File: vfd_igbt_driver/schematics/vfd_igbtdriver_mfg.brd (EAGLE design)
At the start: 160 x 100 mm, 97 parts, among them J1 FS-PW 2,8, J10 FS-PW 2,8, J11 FS-P 6,35, J12 FS-P 6,35, J13 FS-PW 2,8, J14 FS-PW 2,8, J15 FS-PW 2,8, J16 FS-PW 2,8, J17 FS-P 6,35, J18 FS-P 6,35, J19 FS-PW 2,8, J2 FS-PW 2,8, J20 FS-PW 2,8, J21 FS-PW 2,8, J22 FS-PW 2,8, J23 FS-P 6,35, J24 FS-P 6,35, J25 FS-PW 2,8, J26 FS-PW 2,8, J27 FS-PW 2,8, J28 FS-PW 2,8, J29 FS-P 6,35, J3 FS-PW 2,8, J30 FS-P 6,35, J31 FS-PW 2,8, J32 FS-PW 2,8, J33 FS-PW 2,8, J34 FS-PW 2,8, J35 FS-P 6,35, J36 FS-P 6,35, J4 FS-PW 2,8, J5 FS-P 6,35, J6 FS-P 6,35, J7 FS-PW 2,8, J8 FS-PW 2,8, J9 FS-PW 2,8

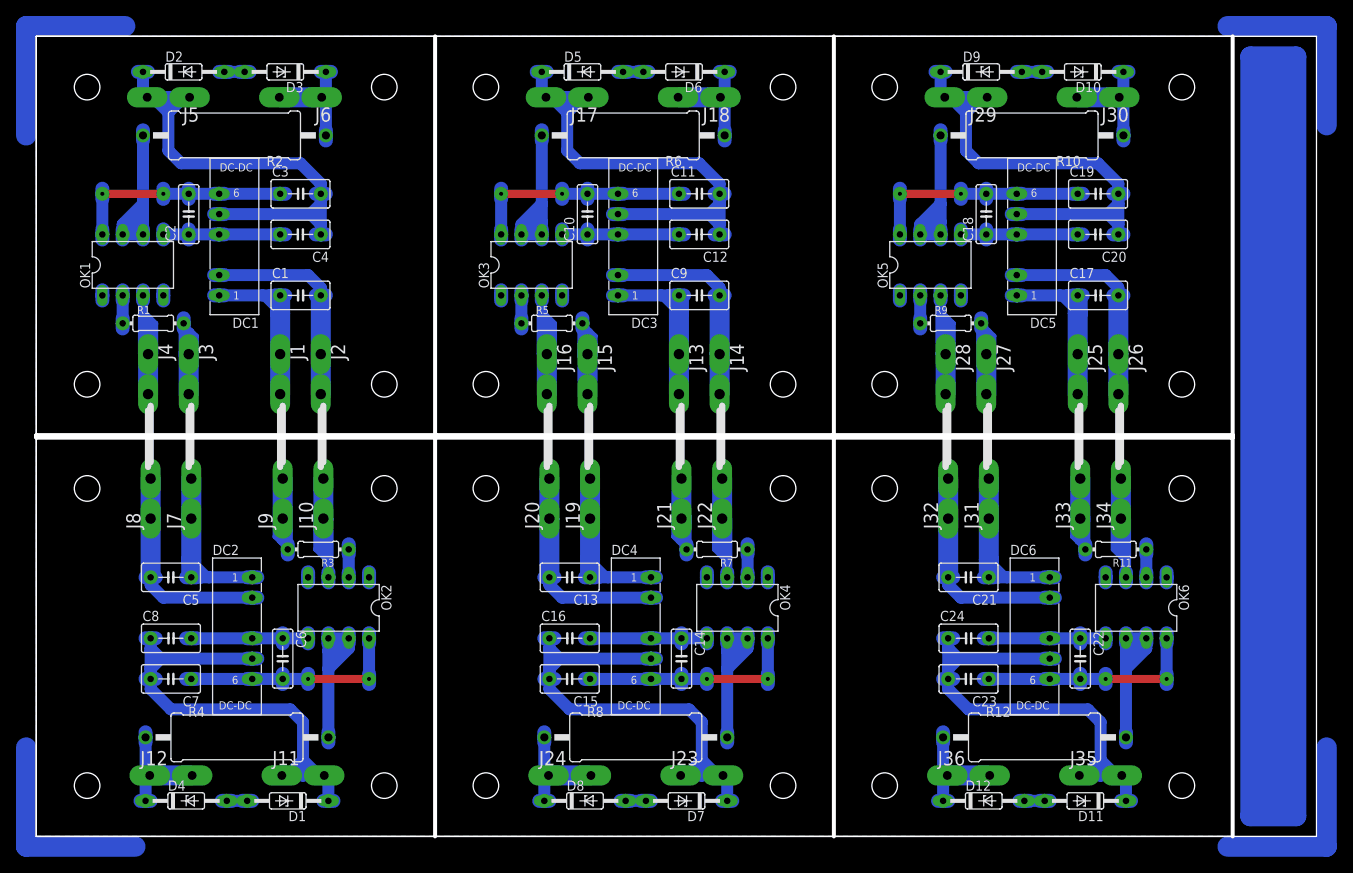
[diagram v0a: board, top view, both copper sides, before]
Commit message: Multiple Changes
Fixed the footprint bug from the igbt drivers

Added schematics and pcb for dc-bus

Added new folders for partial pfc voltage doubling rectifier

Added schematics for controller
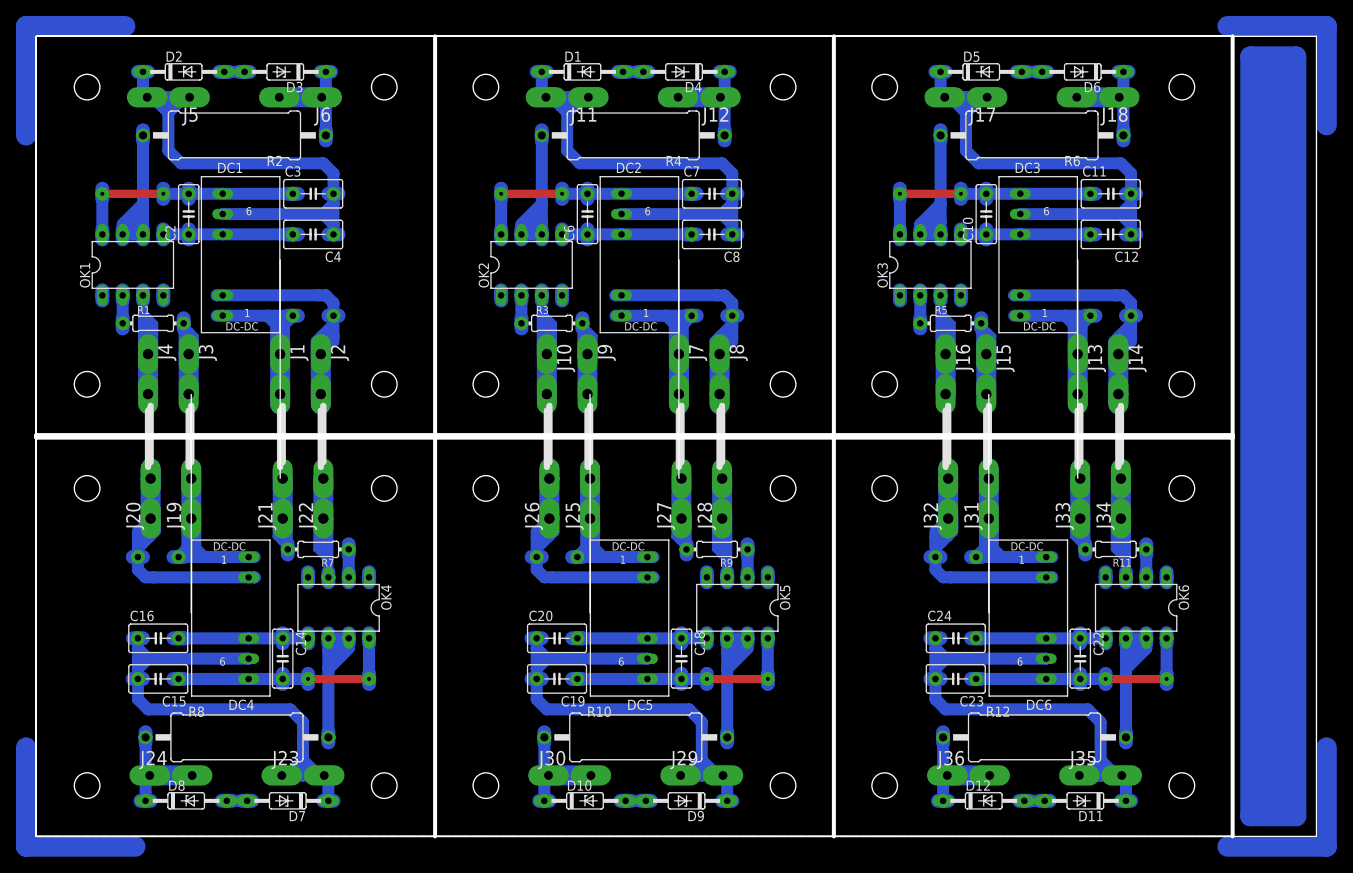
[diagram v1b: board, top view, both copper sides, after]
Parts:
- DC1, DC2, DC3, DC4, DC5, DC6: device dc-dc-converter:NMA -> custom:MGJ2
- moved D10 110.3 mm to (68.6, 4.45), turned to 0 degrees
- moved D4 110.3 mm to (81.0, 95.6), turned to 180 degrees
- moved J12 107.5 mm to (82.9, 92.4), turned to 180 degrees
- moved J30 107.5 mm to (66.7, 7.62), turned to 0 degrees
- moved D1 98.3 mm to (68.3, 95.6), turned to 0 degrees
- moved D9 98.3 mm to (81.3, 4.45), turned to 180 degrees
- moved J11 91.0 mm to (66.4, 92.4), turned to 180 degrees
- moved J29 91.0 mm to (83.2, 7.62), turned to 0 degrees
- moved C19 90.8 mm to (65.1, 19.7), turned to 180 degrees
- moved C7 90.8 mm to (84.5, 80.3), turned to 0 degrees
- moved R4 90.1 mm to (74.6, 87.6), turned to 180 degrees
- moved R10 90.1 mm to (74.9, 12.4), turned to 0 degrees
- moved C20 84.4 mm to (65.1, 24.8), turned to 0 degrees
- moved C8 84.4 mm to (84.5, 75.2), turned to 180 degrees
- moved C17 75.1 mm to (65.1, 34.9), flipped to the bottom
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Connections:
- net EMITTER: now also DC1.6; no longer DC1.5
- net EMITTER1: now also DC2.6; no longer DC2.5
- net EMITTER2: now also DC3.6; no longer DC3.5
- net EMITTER3: now also DC4.6; no longer DC4.5
- net EMITTER4: now also DC5.6; no longer DC5.5
- net EMITTER5: now also DC6.6; no longer DC6.5
- net N$1: now also DC1.5; no longer DC1.4
- net N$15: now also DC3.5; no longer DC3.4
- net N$16: now also DC3.7; no longer DC3.6
- net N$2: now also DC1.7; no longer DC1.6
- net N$22: now also DC4.5; no longer DC4.4
- net N$23: now also DC4.7; no longer DC4.6
- net N$29: now also DC5.5; no longer DC5.4
- net N$30: now also DC5.7; no longer DC5.6
- net N$36: now also DC6.5; no longer DC6.4
- net N$37: now also DC6.7; no longer DC6.6
- net N$7: now also DC2.5; no longer DC2.4
- net N$9: now also DC2.7; no longer DC2.6
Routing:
- net 0V1: track 33.6 -> 39.9 mm, vias 2 -> 1
- net 0V4: track 33.6 -> 39.9 mm, vias 2 -> 1
- net 0V5: track 33.6 -> 39.9 mm, vias 2 -> 1
- net 0V3: track 33.6 -> 39.9 mm, vias 2 -> 1
- net 0V: track 33.6 -> 39.9 mm, vias 2 -> 1
- net 0V2: track 33.6 -> 39.9 mm, vias 2 -> 1
- net EMITTER2: track 73.2 -> 71.1 mm, vias 4 -> 3
- net EMITTER: track 73.2 -> 71.1 mm, vias 4 -> 3
- net EMITTER5: track 73.2 -> 71.1 mm, vias 4 -> 3
- net EMITTER1: track 73.2 -> 71.1 mm, vias 4 -> 3
- net EMITTER3: track 73.2 -> 71.1 mm, vias 4 -> 3
- net EMITTER4: track 73.2 -> 71.1 mm, vias 4 -> 3
- net N$9: track 31.1 -> 32.7 mm, vias 6 -> 5
- net N$16: track 31.1 -> 32.7 mm, vias 6 -> 5
- net N$23: track 31.1 -> 32.7 mm, vias 6 -> 5
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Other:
- outline, holes or cut-outs redrawn

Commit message: Update Controller Schematic & PCB
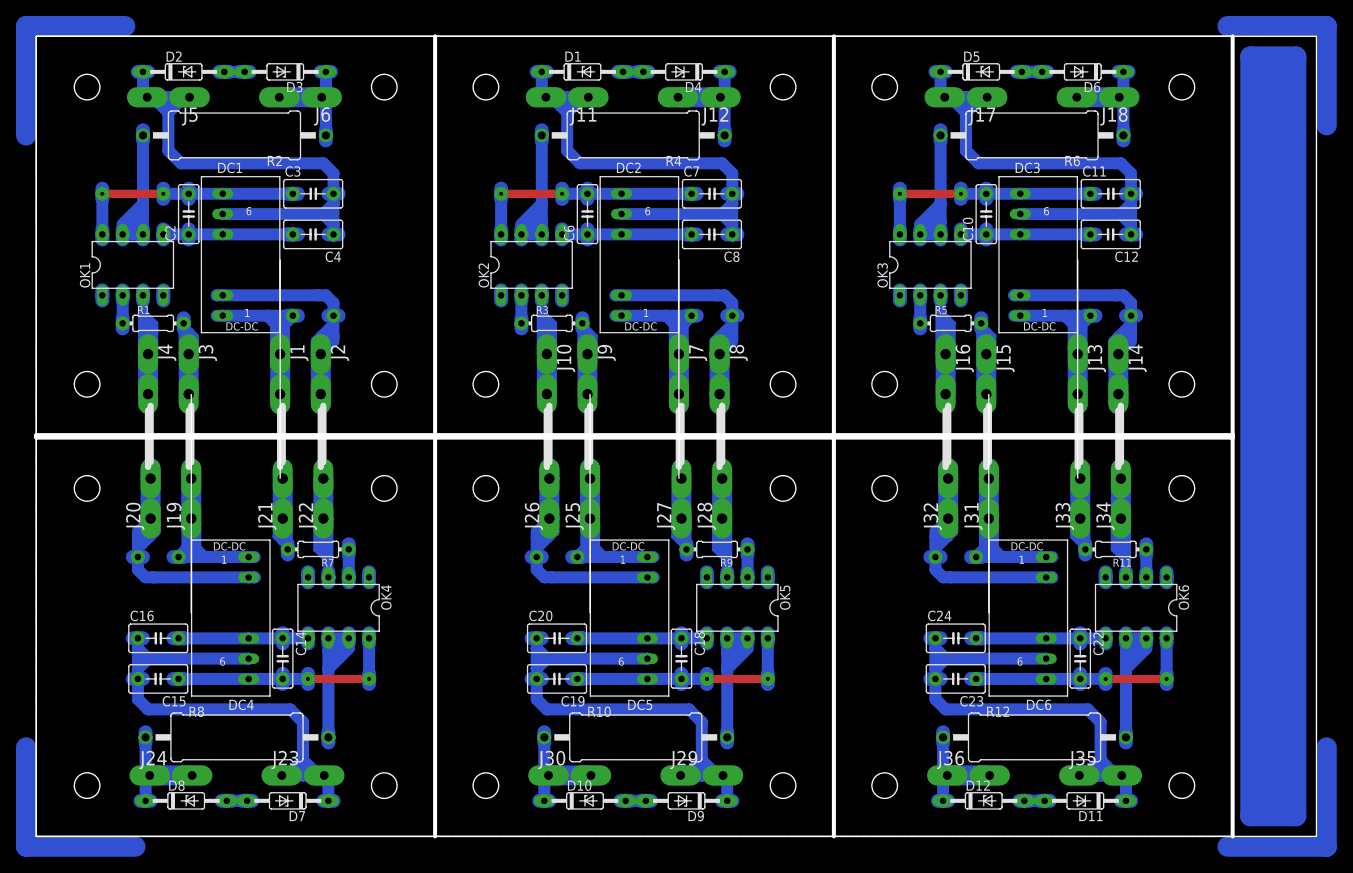
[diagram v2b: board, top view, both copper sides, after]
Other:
- board text added: "(C) 2019 Christoph Klie"
- board text removed: "Christoph Klie"
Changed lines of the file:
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@@
 <wire x1="160.02" y1="0" x2="160.02" y2="100.0125" width="0.1524" layer="20"/>
 <wire x1="160.02" y1="100.0125" x2="0" y2="100.0125" width="0.1524" layer="20"/>
-<wire x1="0" y1="50.165" x2="49.8475" y2="50.165" width="0" layer="20"/>
-<wire x1="0" y1="100.0125" x2="0" y2="50.165" width="0" layer="20"/>
-<wire x1="0" y1="100.0125" x2="49.8475" y2="100.0125" width="0" layer="20"/>
-<wire x1="49.8475" y1="49.8475" x2="0" y2="49.8475" width="0" layer="20"/>
-<wire x1="49.8475" y1="0" x2="0" y2="0" width="0" layer="20"/>
-<wire x1="0" y1="0" x2="0" y2="49.8475" width="0" layer="20"/>
-<wire x1="49.8475" y1="50.165" x2="99.695" y2="50.165" width="0" layer="20"/>
-<wire x1="49.8475" y1="100.0125" x2="49.8475" y2="50.165" width="0" layer="20"/>
-<wire x1="49.8475" y1="100.0125" x2="99.695" y2="100.0125" width="0" layer="20"/>
-<wire x1="99.695" y1="49.8475" x2="49.8475" y2="49.8475" width="0" layer="20"/>
-<wire x1="99.695" y1="0" x2="49.8475" y2="0" width="0" layer="20"/>
-<wire x1="49.8475" y1="0" x2="49.8475" y2="49.8475" width="0" layer="20"/>
-<wire x1="99.695" y1="50.165" x2="149.5425" y2="50.165" width="0" layer="20"/>
-<wire x1="99.695" y1="100.0125" x2="99.695" y2="50.165" width="0" layer="20"/>
-<wire x1="99.695" y1="100.0125" x2="149.5425" y2="100.0125" width="0" layer="20"/>
-<wire x1="149.5425" y1="100.0125" x2="149.5425" y2="50.165" width="0" layer="20"/>
-<wire x1="149.5425" y1="49.8475" x2="99.695" y2="49.8475" width="0" layer="20"/>
-<wire x1="149.5425" y1="0" x2="149.5425" y2="49.8475" width="0" layer="20"/>
-<wire x1="149.5425" y1="0" x2="99.695" y2="0" width="0" layer="20"/>
-<wire x1="99.695" y1="0" x2="99.695" y2="49.8475" width="0" layer="20"/>
-<text x="128.5875" y="-33.3375" size="2.54" layer="48">Christoph Klie</text>
-<text x="130.175" y="-28.2575" size="2.54" layer="48">IGBT-Driver</text>
-<text x="120.65" y="-23.1775" size="2.54" layer="48">Variable Frequency Drive</text>
+<text x="122.39625" y="-33.3375" size="2.54" layer="48">(C) 2019 Christoph Klie</text>
+<text x="131.6880875" y="-28.2575" size="2.54" layer="48">IGBT-Driver</text>
+<text x="120.91455625" y="-23.1775" size="2.54" layer="48">Variable Frequency Drive</text>
 <text x="169.545" y="-36.195" size="2.54" layer="48">Version 1.0</text>
 <text x="200.3425" y="-36.195" size="2.54" layer="48">[1/1]</text>
@@
 <hole x="43.4975" y="93.6625" drill="3.2"/>
 <hole x="43.4975" y="56.515" drill="3.2"/>
-<wire x1="49.8475" y1="100.0125" x2="49.8475" y2="50.165" width="0" layer="20"/>
 <polygon width="0.0254" layer="42">
 <vertex x="6.6675" y="73.3425"/>
@@
 <hole x="93.345" y="93.6625" drill="3.2"/>
 <hole x="93.345" y="56.515" drill="3.2"/>
-<wire x1="99.695" y1="100.0125" x2="99.695" y2="50.165" width="0" layer="20"/>
 <polygon width="0.0254" layer="42">
 <vertex x="56.515" y="73.3425"/>
@@
 <wire x1="49.8475" y1="49.8475" x2="0" y2="49.8475" width="0" layer="20"/>
 <hole x="43.4975" y="6.35" drill="3.2"/>
-<wire x1="49.8475" y1="0" x2="49.8475" y2="49.8475" width="0" layer="20"/>
 <wire x1="49.8475" y1="0" x2="0" y2="0" width="0" layer="20"/>
 <hole x="43.4975" y="43.4975" drill="3.2"/>
@@
 <wire x1="99.695" y1="49.8475" x2="49.8475" y2="49.8475" width="0" layer="20"/>
 <hole x="93.345" y="6.35" drill="3.2"/>
-<wire x1="99.695" y1="0" x2="99.695" y2="49.8475" width="0" layer="20"/>
 <wire x1="99.695" y1="0" x2="49.8475" y2="0" width="0" layer="20"/>
 <hole x="93.345" y="43.4975" drill="3.2"/>
